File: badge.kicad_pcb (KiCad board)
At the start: 2 copper layers, 76.2 x 127 mm, 1 part

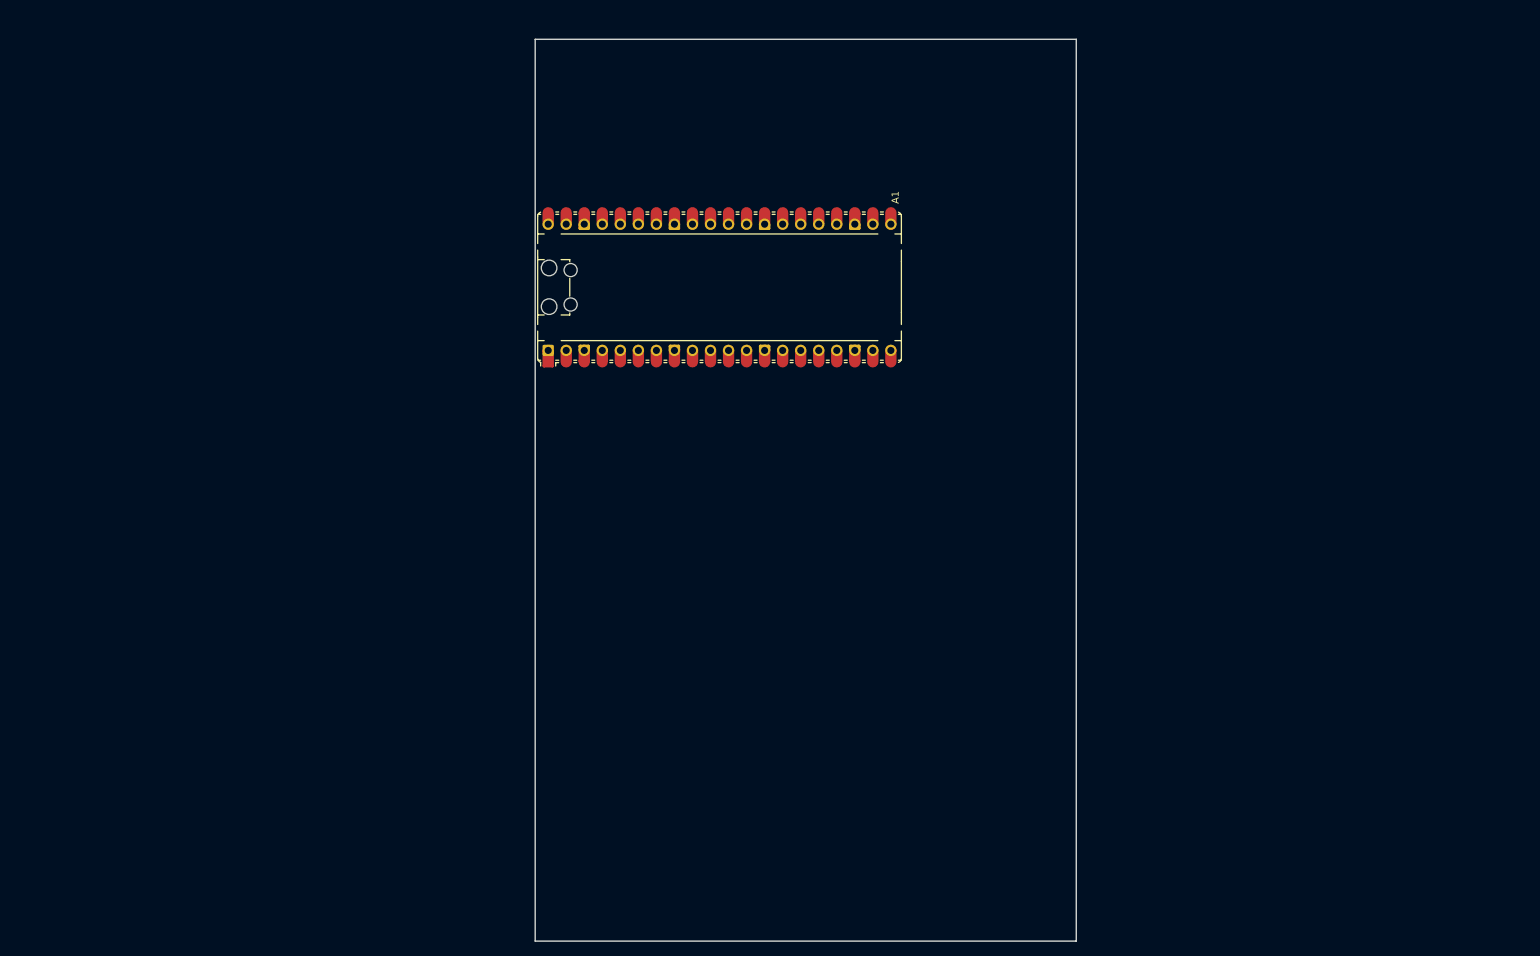
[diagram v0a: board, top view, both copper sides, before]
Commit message: now we start layout
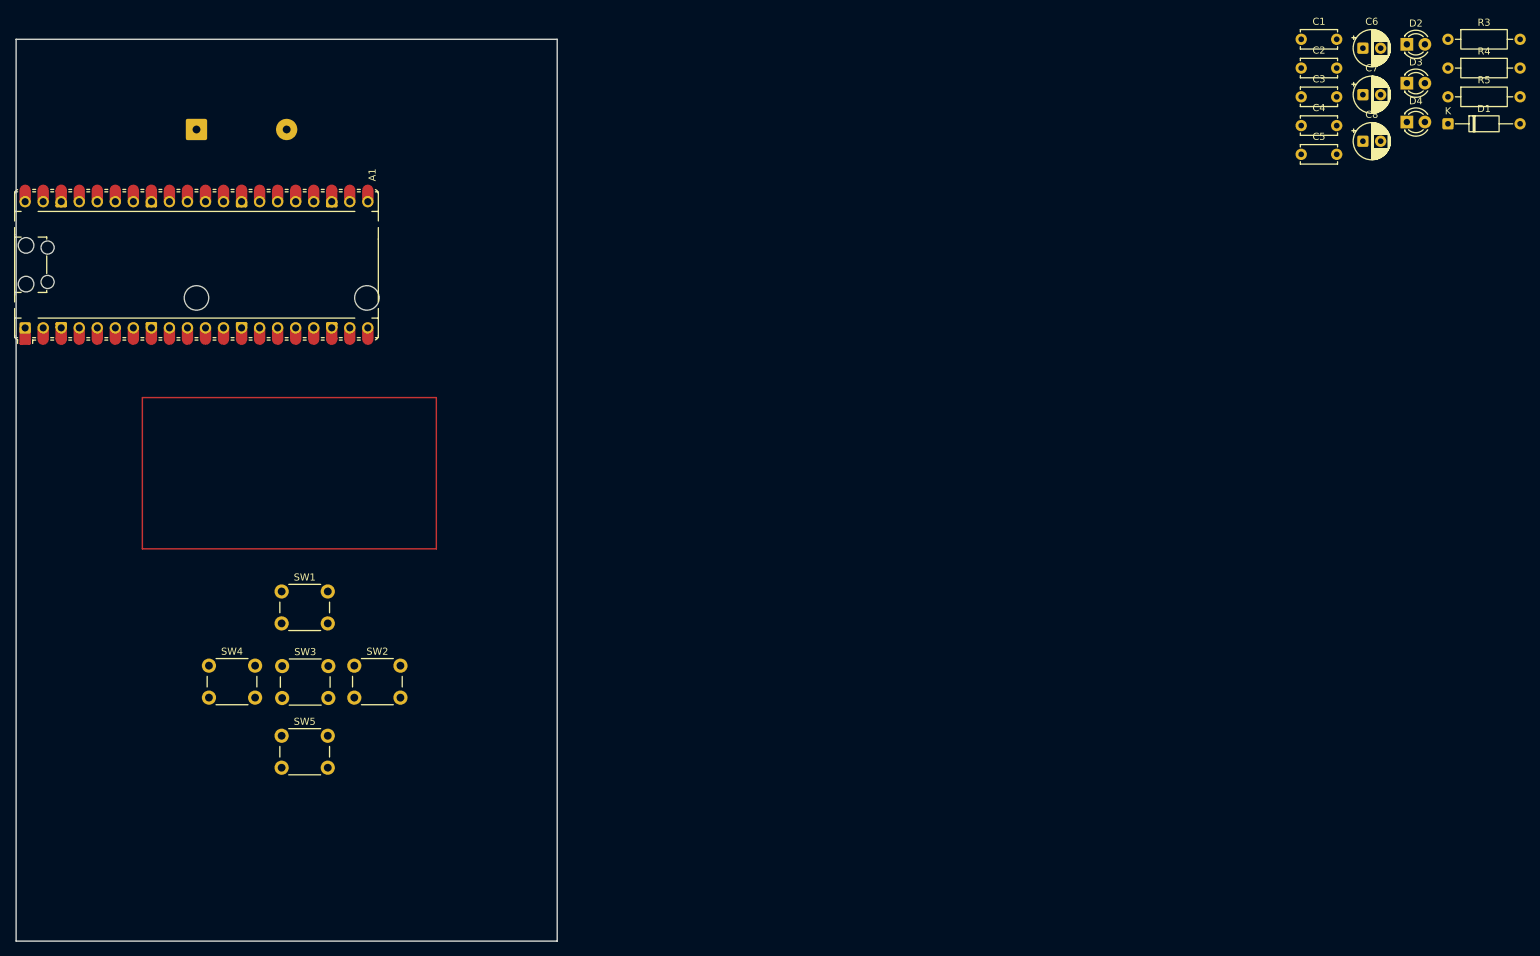
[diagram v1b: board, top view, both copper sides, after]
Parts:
- added BT1: Battery_Cell, Battery:BatteryHolder_Keystone_2479_3xAAA, B.Cu at (50.8, 38.1)
- added C1: C, Capacitor_THT:C_Disc_D5.0mm_W2.5mm_P5.00mm, F.Cu at (206.4, 25.4)
- added C2: C, Capacitor_THT:C_Disc_D5.0mm_W2.5mm_P5.00mm, F.Cu at (206.4, 29.4)
- added C3: C, Capacitor_THT:C_Disc_D5.0mm_W2.5mm_P5.00mm, F.Cu at (206.4, 33.5)
- added C4: C, Capacitor_THT:C_Disc_D5.0mm_W2.5mm_P5.00mm, F.Cu at (206.4, 37.5)
- added C5: C, Capacitor_THT:C_Disc_D5.0mm_W2.5mm_P5.00mm, F.Cu at (206.4, 41.6)
- added C6: C, Capacitor_THT:CP_Radial_D5.0mm_P2.50mm, F.Cu at (215.1, 26.6)
- added C7: C, Capacitor_THT:CP_Radial_D5.0mm_P2.50mm, F.Cu at (215.1, 33.2)
- added C8: C, Capacitor_THT:CP_Radial_D5.0mm_P2.50mm, F.Cu at (215.1, 39.8)
- added D1: D_Schottky, Diode_THT:D_DO-35_SOD27_P10.16mm_Horizontal, F.Cu at (227.0, 37.3)
- added D2: LED, LED_THT:LED_D3.0mm, F.Cu at (221.3, 26.1)
- added D3: LED, LED_THT:LED_D3.0mm, F.Cu at (221.3, 31.6)
- added D4: LED, LED_THT:LED_D3.0mm, F.Cu at (221.3, 37.0)
- added R3: R, Resistor_THT:R_Axial_DIN0207_L6.3mm_D2.5mm_P10.16mm_Horizontal, F.Cu at (227.0, 25.4)
- added R4: R, Resistor_THT:R_Axial_DIN0207_L6.3mm_D2.5mm_P10.16mm_Horizontal, F.Cu at (227.0, 29.4)
- added R5: R, Resistor_THT:R_Axial_DIN0207_L6.3mm_D2.5mm_P10.16mm_Horizontal, F.Cu at (227.0, 33.5)
- added SW1: SW_Push, Button_Switch_THT:SW_PUSH_6mm, F.Cu at (62.8, 103.2)
- added SW2: SW_Push, Button_Switch_THT:SW_PUSH_6mm, F.Cu at (73.0, 113.6)
- added SW3: SW_Push, Button_Switch_THT:SW_PUSH_6mm, F.Cu at (62.9, 113.7)
- added SW4: SW_Push, Button_Switch_THT:SW_PUSH_6mm, F.Cu at (52.6, 113.6)
- added SW5: SW_Push, Button_Switch_THT:SW_PUSH_6mm, F.Cu at (62.8, 123.5)
- moved A1 73.7 mm to (50.8, 57.1)
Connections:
- A1 pad 10: unconnected-(A1-GPIO7-Pad10) -> Net-(A1-GPIO7)
- A1 pad 12: unconnected-(A1-GPIO9-Pad12) -> Net-(A1-GPIO9)
- A1 pad 14: unconnected-(A1-GPIO10-Pad14) -> Net-(A1-GPIO10)
- A1 pad 15: unconnected-(A1-GPIO11-Pad15) -> Net-(A1-GPIO11)
- A1 pad 16: unconnected-(A1-GPIO12-Pad16) -> Net-(A1-GPIO12)
- A1 pad 17: unconnected-(A1-GPIO13-Pad17) -> Net-(A1-GPIO13)
- A1 pad 2: Net-(A1-GPIO1) -> unconnected-(A1-GPIO1-Pad2)
- A1 pad 21: unconnected-(A1-GPIO16-Pad21) -> Net-(A1-GPIO16)
- A1 pad 22: unconnected-(A1-GPIO17-Pad22) -> Net-(A1-GPIO17)
- A1 pad 24: unconnected-(A1-GPIO18-Pad24) -> Net-(A1-GPIO18)
- A1 pad 4: Net-(A1-GPIO2) -> unconnected-(A1-GPIO2-Pad4)
- A1 pad 5: Net-(A1-GPIO3) -> unconnected-(A1-GPIO3-Pad5)

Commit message: work has been proceding
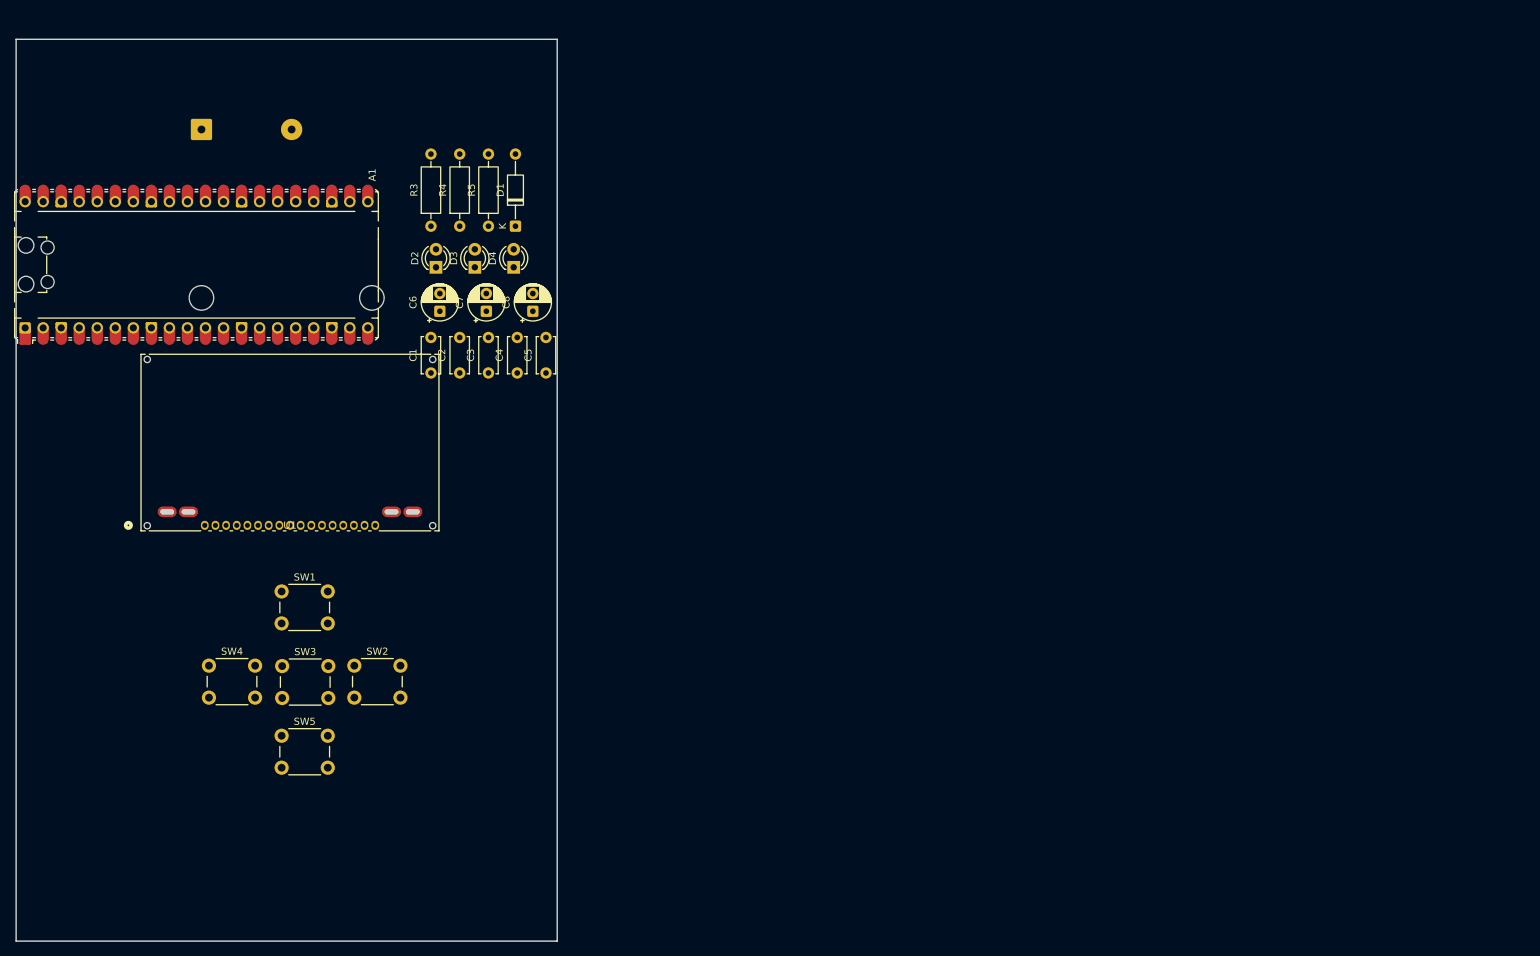
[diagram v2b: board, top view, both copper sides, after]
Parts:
- added U1: NHD-C12832A1Z-FSRGB-FBW-3V, FTbadge:NHD-C12_NDI, F.Cu at (52.0, 93.8)
- moved R3 145.6 mm to (83.8, 51.7), turned to 90 degrees
- moved R4 140.9 mm to (87.9, 51.7), turned to 90 degrees
- moved D2 140.3 mm to (84.5, 57.5), turned to 90 degrees
- moved R5 136.3 mm to (91.9, 51.7), turned to 90 degrees
- moved C6 135.2 mm to (85.1, 63.7), turned to 90 degrees
- moved D3 133.8 mm to (90.0, 57.5), turned to 90 degrees
- moved D1 132.1 mm to (95.7, 51.7), turned to 90 degrees
- moved C1 131.3 mm to (83.8, 72.4), turned to 90 degrees
- moved D4 127.4 mm to (95.5, 57.5), turned to 90 degrees
- moved C7 127.2 mm to (91.6, 63.7), turned to 90 degrees
- moved C2 126.0 mm to (87.9, 72.4), turned to 90 degrees
- moved C3 120.9 mm to (91.9, 72.4), turned to 90 degrees
- moved C8 119.3 mm to (98.2, 63.7), turned to 90 degrees
- moved C4 115.8 mm to (96.0, 72.4), turned to 90 degrees
- moved C5 110.7 mm to (100.0, 72.4), turned to 90 degrees
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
